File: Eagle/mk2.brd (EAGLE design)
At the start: 100 x 75 mm, 87 parts, among them Q1 BC847B, SW1 EVQQ2, SW2 MFP106D, U1 TPS63061DSCT, U2 TPS63061DSCT, U3 DRV8833PWPR, U4 TCA9406DCTR, U5 MPU-6050, U6 74AHCT1G32GW/T1, U7 ATMEGA328-AU

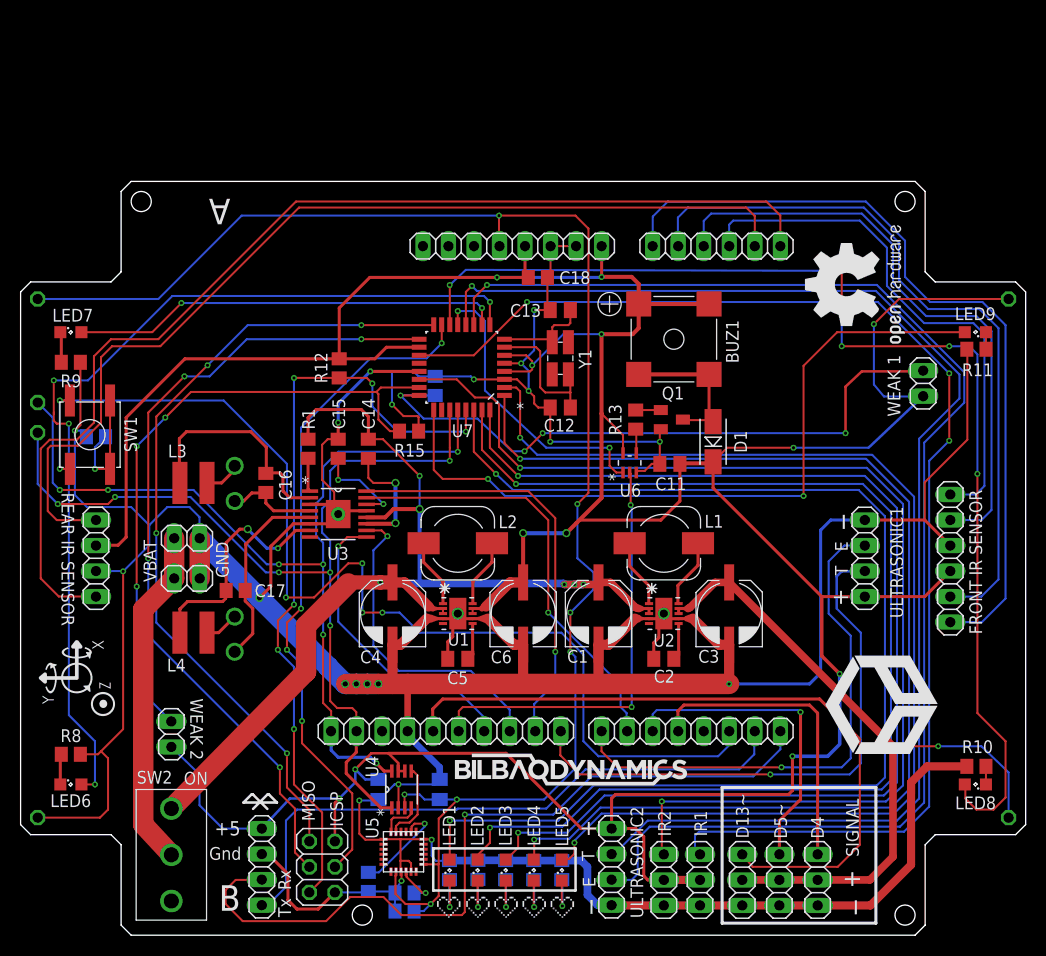
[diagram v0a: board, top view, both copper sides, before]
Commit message: update
files
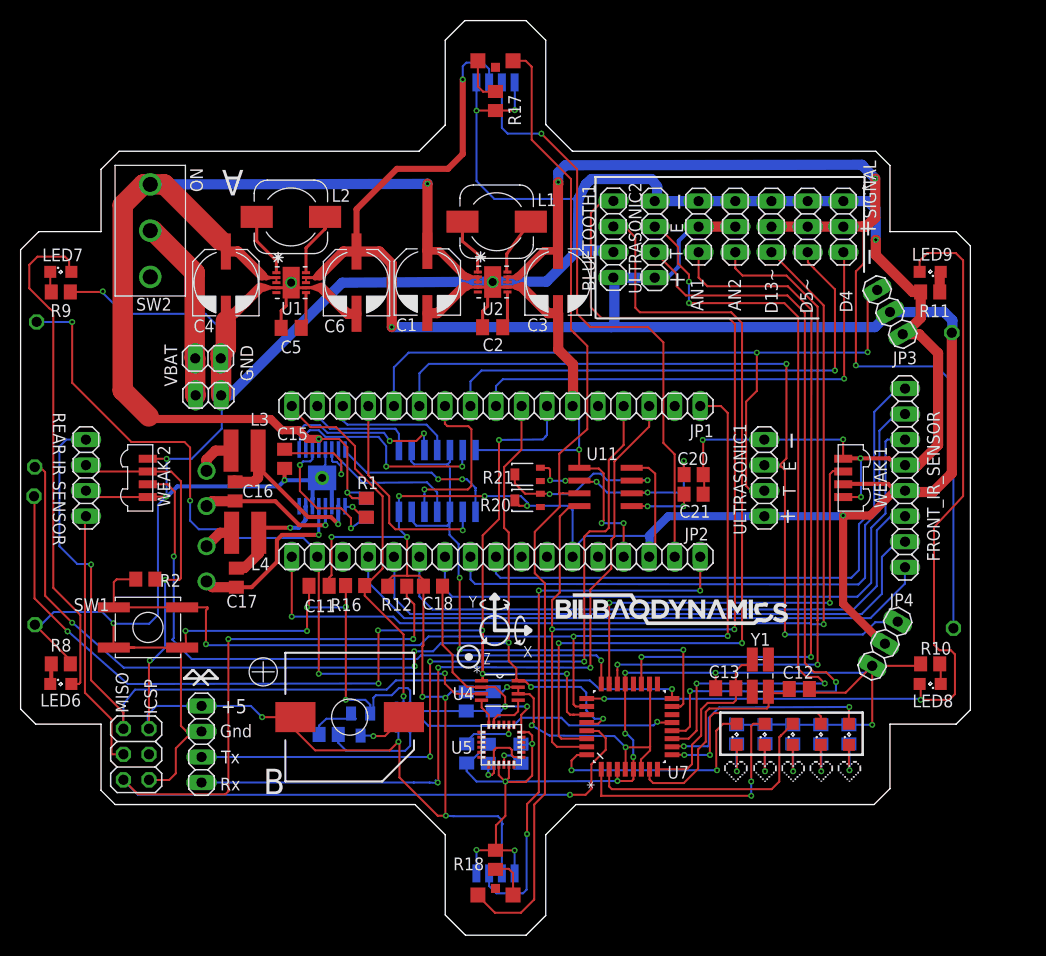
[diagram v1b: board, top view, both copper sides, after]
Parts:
- removed BUZ1: KSSG74B16, Jaegger_MKII:KSSG74B16
- removed D1: S1B-13-F, Jaegger_MKII:S1B-13-F
- removed IR1: SHARP GP2Y0A21YK, pinhead:1X03
- removed IR2: SHARP GP2Y0A21YK3, pinhead:1X03
- removed JP6, JP7: (no value), pinhead:1X02
- removed R14, R15: 10k, resistor:R0805
- added AN1: SHARP GP2Y0A21YK, pinhead:1X03
- added AN2: SHARP GP2Y0A21YK3, pinhead:1X03
- added BLUETOOTH1: HC-06 Female Header, pinhead:1X04
- added BUZZ1: KTG1205C, Jaegger_MKII:KTG1205C
- added C20, C21: 0.1µF, rcl:C0805
- added IR_REC1, IR_REC2, IR_REC3, IR_REC4: TSMP77000TR, Jaegger_MKII:TSMP77000TR
- added R16: 10k, rcl:R0805
- added R17, R18: 1k, rcl:R0805
- added R20, R21: 20KOHM, Panasonic-Trimmer_Potentiometers:POT_EVM2N
- added U$1, U$2: KPA-3010F3C, Jaegger_MKII:KPA-3010F3C
- added U11: UA555D, linear:SO08
- added U8: 74ALS08D, 74xx-eu:SO14
- C10: value 0.1µF -> 2.2nF; device rcl:C0805K -> rcl:C0805
- C19: value 2.2nF -> 0.1µF
- C7: value 0.1uF -> 0.1µF
- C9: device rcl:C0805K -> rcl:C0805
- FRONT_IR_SENSOR: device pinhead:1X06 -> pinhead:1X08
- JP1: value Arduino Leonardo -> (none); device pinhead:1X08 -> pinhead:1X17
- JP2: value Arduino Leonardo -> (none); device pinhead:1X10 -> pinhead:1X17
- JP3: value Arduino Leonardo -> IR1; device pinhead:1X08 -> pinhead:1X03
- JP4: value Arduino Leonardo -> IR2; device pinhead:1X06 -> pinhead:1X03
- R10, R11, R8, R9: value 330 -> 1k
- R2: value 330 -> 10k
- U4: device texas:SOP65P400X130-8N -> TCA9406DCTR:SOP65P400X130-8N
- moved D13~ 65.1 mm to (74.7, 70.5), turned to 90 degrees
- moved D5~ 65.1 mm to (78.3, 70.5), turned to 90 degrees
- moved D4 65.1 mm to (81.9, 70.5), turned to 90 degrees
- moved ULTRASONIC2 62.6 mm to (63.1, 69.2), turned to 90 degrees
- moved SW2 62.1 mm to (12.9, 70.1)
- moved JP3 46.2 mm to (86.5, 62.0), turned to 300 degrees
- moved R13 43.8 mm to (30.7, 20.0), flipped to the bottom, turned to 180 degrees
- moved Q1 43.4 mm to (33.8, 21.0), flipped to the bottom, turned to 180 degrees
- moved JP4 43.0 mm to (86.0, 29.0), turned to 240 degrees
- moved C13 41.1 mm to (70.2, 24.6)
- moved U7 39.4 mm to (60.6, 20.8), turned to 90 degrees
- moved Y1 37.3 mm to (73.6, 25.8)
- moved C1 37.1 mm to (40.5, 65.0)
- moved C3 37.1 mm to (53.5, 65.0)
- moved U2 37.1 mm to (47.0, 65.0)
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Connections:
- removed net ADC6: IR1.1, U7.19
- removed net ADC7: IR2.1, U7.22
- removed net AN3: U7.26
- removed net BUTTON: JP3.6, SW1.P$2, SW1.P$3
- removed net BUZZER_ARDUINO: JP2.6, U6.2
- removed net CAÑON: D4.1, JP3.4
- removed net ECHO_ARDUINO: JP3.1, ULTRASONIC1.3
- removed net ILUM_3: LED8.A, U7.14
- removed net ILUM_4: LED9.A, U7.25
- removed net MISO: ICSP.1, U7.16
- removed net SERVO1: D13~.1, JP2.5
- removed net SERVO2: D5~.1, JP3.3
- removed net TRIGGER_ARDUINO: JP2.10, ULTRASONIC1.2
- new net ADC6_EXT: AN1.1, U7.19
- new net ADC7_EXT: AN2.1, U7.22
- new net BUTTON/D16/328: JP1.1, R2.2, SW1.P$1, SW1.P$4, U7.26
- new net D10/BIN2: JP1.15, U8.4
- new net D11/BIN1: JP1.16, U8.1
- new net D12/BUZZER_ARDUINO: JP1.17, R16.1, U6.2
- new net D13/SERVO1: D13~.1, JP2.17
- new net D14/MISO_MICRO: IR_REC1.3, JP2.2
- new net D15/SCK_MICRO: IR_REC2.3, JP2.1
- new net D4/CAÑON: D4.1, JP1.9
- new net D5/SERVO2: D5~.1, JP1.10
- new net D6/AIN2: JP1.11, U8.12
- new net D7/ECHO_ARDUINO: JP1.12, JP4.1, ULTRASONIC1.3
- new net D8/TRIGGER_ARDUINO: JP1.13, JP3.1, ULTRASONIC1.2
- new net D9/AIN1: JP1.14, U8.9
- new net ILUM1: U7.14
- new net MISO/IR_REAR_LEFT: BACK_IR_SENSOR.4, ICSP.1, U7.16
- new net MOSI/ENABLE: U7.15, U8.10, U8.13, U8.2, U8.5
- new net N$35: C10.1, U5.20
- new net N$36: C9.1, U5.10
- new net N$39: R20.3, R21.2, U11.7
- new net N$40: R18.1, U$2.C
- new net N$42: C21.1, U11.5
- new net OUTPUT_555: U$1.A, U$2.A, U11.3
- new net RX328: BLUETOOTH1.3, U7.30
- new net SCK/IR_REAR_RIGHT: U7.17
- new net TX328/ENABLE555: BLUETOOTH1.4, U11.4, U7.31
- net +3V3: now also JP2.16; no longer C10.1, C7.1, JP1.4, U5.13, U5.8
- net +5V_CONTROL: now also AN1.2, AN2.2, BLUETOOTH1.1, BUZZ1.+, C7.1, C8.1, IR_REC1.2, IR_REC2.2, IR_REC3.2, IR_REC4.2, JP2.3, JP2.6, JP3.2, JP4.2, R2.1, R20.2, U11.8, U8.14; no longer BUZ1.P$2, BUZ1.P$3, C9.1, D1.2, IR1.2, IR2.2, JP1.5, JP1.8, JP6.1, JP7.1
- net A0: now also FRONT_IR_SENSOR.1, JP2.14; no longer FRONT_IR_SENSOR.6, JP4.1
- net A1: now also FRONT_IR_SENSOR.2, JP2.13; no longer FRONT_IR_SENSOR.5, JP4.2
- net A2: now also FRONT_IR_SENSOR.3, JP2.12; no longer FRONT_IR_SENSOR.2, JP4.3
- net A3: now also FRONT_IR_SENSOR.6, JP2.11; no longer FRONT_IR_SENSOR.1, JP4.4
- net A4: now also FRONT_IR_SENSOR.7, JP2.10; no longer BACK_IR_SENSOR.4, JP4.5
- net A5: now also FRONT_IR_SENSOR.8, JP2.9; no longer BACK_IR_SENSOR.1, JP4.6
- net AIN1: now also U8.8; no longer JP2.9
- net AIN2: now also U8.11; no longer JP3.2
- net BIN1: now also U8.3; no longer JP2.7
- net BIN2: now also U8.6; no longer JP2.8
- net D0/RX: now also JP1.4; no longer JP3.8
- net D1/TX: now also JP1.3; no longer JP3.7
- net DEBIL_1: now also IR_REC3.3; no longer JP7.2, R15.2
- net DEBIL_2: now also IR_REC4.3; no longer JP6.2, R14.2
- net GND: now also AN1.3, AN2.3, BLUETOOTH1.2, C20.2, C21.2, FRONT_IR_SENSOR.5, IR_REC1.1, IR_REC1.4, IR_REC2.1, IR_REC2.4, IR_REC3.1, IR_REC3.4, IR_REC4.1, IR_REC4.4, JP3.3, JP4.3, R16.2, R17.2, R18.2, SW1.P$2, SW1.P$3, U11.1, U8.7; no longer FRONT_IR_SENSOR.3, IR1.3, IR2.3, JP1.7, R14.1, R15.1, R2.1, U5.1
- net ILUM_1: now also LED7.A; no longer U7.9
- net ILUM_2: now also LED8.A, LED9.A, U7.25; no longer LED7.A, U7.10
- net MOSI: no longer U7.15
- net N$17: now also BUZZ1.-; no longer BUZ1.P$1, BUZ1.P$4, D1.1
- net N$23: now also R17.1, U$1.C; no longer R2.2, SW1.P$1, SW1.P$4
- net N$31: now also C20.1, R21.3, U11.2, U11.6; no longer C8.1, U5.10
- net N$5: now also U5.13, U5.8; no longer U5.20
- net SCK: now also BACK_IR_SENSOR.1; no longer U7.17
- net SCL_5: now also JP1.8; no longer JP2.1
- net SDA_5: now also JP1.7; no longer JP2.2
- net VIDA_1: now also U7.32; no longer U7.30
- net VIDA_2: now also U7.1; no longer U7.31
- net VIDA_3: now also U7.2; no longer U7.32
- net VIDA_4: now also U7.9; no longer U7.1
- net VIDA_5: now also U7.10; no longer U7.2
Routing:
- net ADC6: track 128.6 -> 0.00 mm, vias 3 -> 0
- net ILUM_3: track 116.5 -> 0.00 mm, vias 6 -> 0
- net ADC7: track 113.8 -> 0.00 mm, vias 2 -> 0
- net BUTTON: track 111.1 -> 0.00 mm, vias 6 -> 0
- net TX328/ENABLE555: track 0.00 -> 105.4 mm, vias 0 -> 2
- net BUTTON/D16/328: track 0.00 -> 103.6 mm, vias 0 -> 3
- net GND: track 496.4 -> 599.0 mm, vias 24 -> 35
- net OUTPUT_555: track 0.00 -> 99.4 mm
- net VIDA_1: track 122.6 -> 23.6 mm
- net D13/SERVO1: track 0.00 -> 98.3 mm, vias 0 -> 2
- net VIDA_4: track 117.4 -> 19.7 mm
- net MISO/IR_REAR_LEFT: track 0.00 -> 94.0 mm, vias 0 -> 2
- net VIDA_5: track 116.1 -> 22.5 mm
- net VIDA_2: track 119.4 -> 26.0 mm
- net VIDA_3: track 117.0 -> 25.4 mm, vias 2 -> 0
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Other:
- board size 100 x 75 mm -> 94.5 x 91 mm
- board text added: "BD Robotics Jaeger MKII 2015 bilbaodynamics.com DESIGNED IN EUSKADI MEKAGÜENLAOSTIA"
- board text removed: "BD Robotics Jaeger MKII 2015 bilbaodynamics.com"
- board text removed: "FRONT IR SENSOR"
